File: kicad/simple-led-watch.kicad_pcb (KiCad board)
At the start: 4 copper layers, 32.8 x 32.6 mm, 169 parts, among them P1 BATTERY, P2 SWD, P3 USB_OTG, Q1 MMBT3904, Q2 MMBT3904, SW1 SPST-4PIN, SW2 SPST-4PIN, SW3 SPST-4PIN, SW4 SPST-4PIN, U1 MCP73832, U2 TPS62736, U3 STM32L052CxTx, U4 MMA8652FC, U5 USBLC6-2, U6 74HC154, Y1 32.767KHz

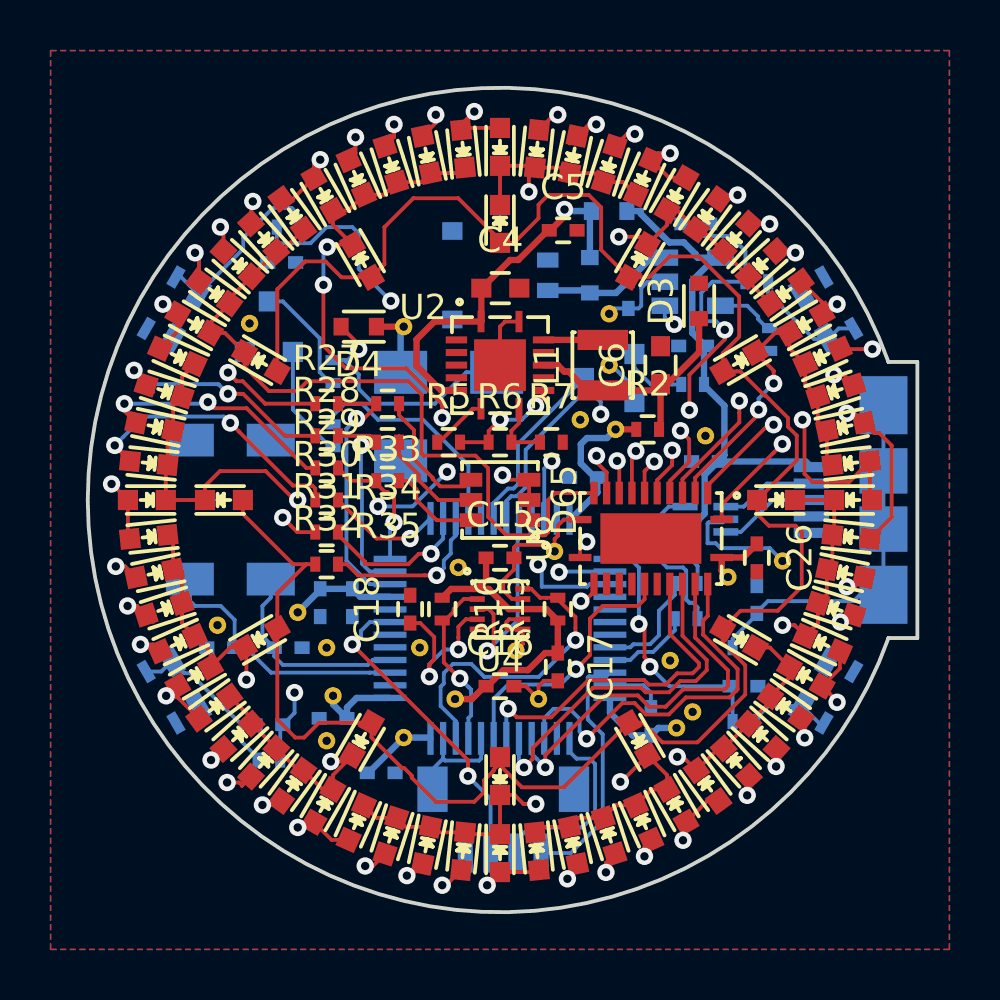
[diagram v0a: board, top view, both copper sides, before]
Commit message: Placed parts for round two
I'm pretty sure I can do it better
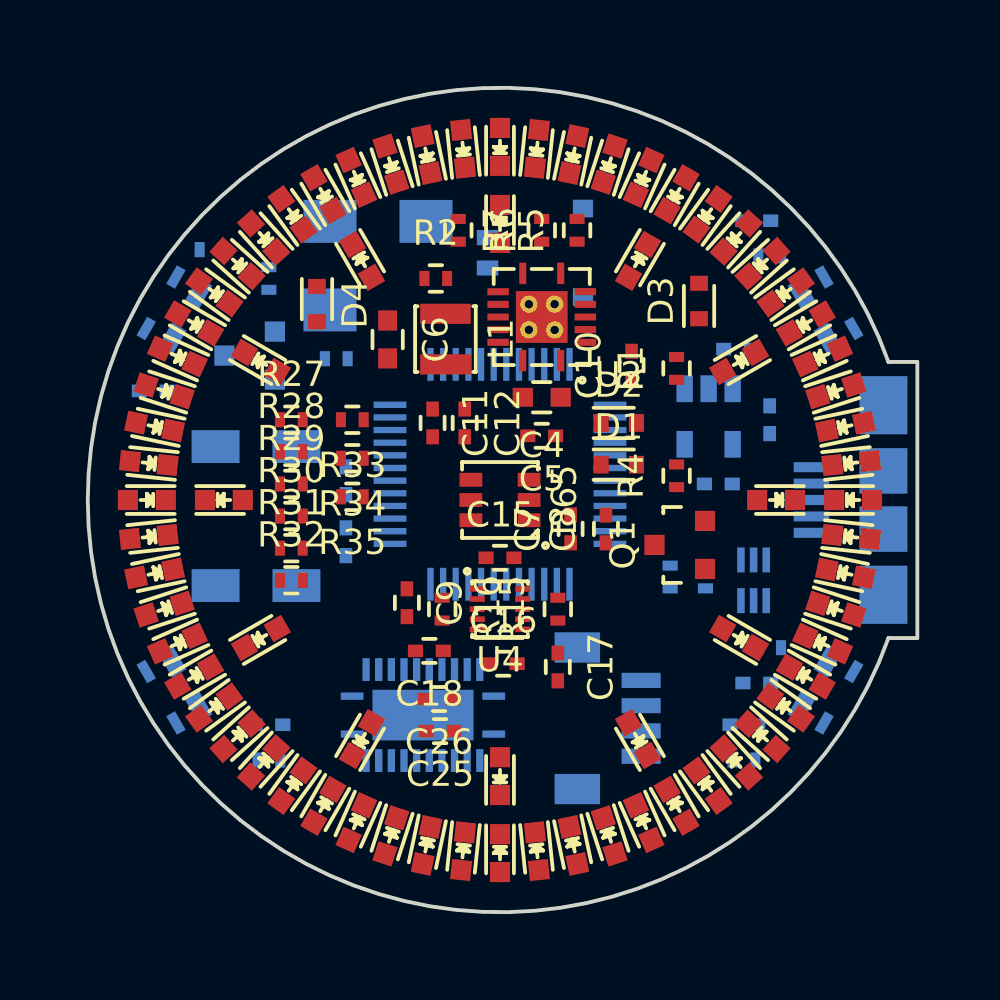
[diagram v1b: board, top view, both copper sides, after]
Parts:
- removed the REF** at (173.2, 86.4)
- removed the REF** at (165.7, 94.9)
- removed the REF** at (169.4, 81.5)
- removed the REF** at (169.4, 83.6)
- removed the REF** at (168.3, 85.7)
- removed the REF** at (176.3, 91.3)
- removed the REF** at (167.3, 90.9)
- removed the REF** at (158.2, 94.7)
- removed the REF** at (169.7, 86.1)
- removed the REF** at (172.1, 97.9)
- removed the REF** at (161.3, 98.3)
- removed the REF** at (166.6, 96.8)
- removed the REF** at (158.5, 96.6)
- removed the REF** at (163.3, 96.8)
- removed the REF** at (157.1, 93.3)
- removed the REF** at (174.1, 91.9)
- removed the REF** at (161.3, 82.0)
- removed the REF** at (161.9, 94.7)
- removed the REF** at (153.9, 93.9)
- removed the REF** at (158.2, 98.4)
- removed the REF** at (155.2, 81.9)
- removed the REF** at (172.7, 97.3)
- removed the REF** at (171.8, 95.2)
- removed the REF** at (163.4, 91.6)
- added C25: 1u, Capacitors_SMD:C_0402, F.Cu at (162.7, 98.0)
- added REF**: 1PIN_VIA, simple-led-watch:1PIN_VIA, F.Cu at (167.3, 82.2)
- added REF**: 1PIN_VIA, simple-led-watch:1PIN_VIA, F.Cu at (166.2, 82.2)
- added REF**: 1PIN_VIA, simple-led-watch:1PIN_VIA, F.Cu at (166.2, 81.2)
- added REF**: 1PIN_VIA, simple-led-watch:1PIN_VIA, F.Cu at (167.3, 81.2)
- C10, C11, C12, C7, C8, C9, D1, D2, Q1, R1, R4: moved to F.Cu
- U6: moved to B.Cu
- moved C10 18.9 mm to (170.3, 83.6), turned to 90 degrees
- moved C26 13.8 mm to (162.7, 96.8), turned to 180 degrees
- moved U6 11.4 mm to (162.1, 97.4)
- moved C6 10.8 mm to (160.7, 82.5), turned to 270 degrees
- moved R2 10.3 mm to (162.6, 80.1)
- moved D1 10.0 mm to (169.8, 87.5)
- moved R5 9.80 mm to (168.1, 78.2), turned to 90 degrees
- moved C12 9.12 mm to (163.7, 85.9)
- moved R6 8.54 mm to (163.4, 78.2), turned to 270 degrees
- moved R7 8.39 mm to (166.8, 78.2), turned to 90 degrees
- moved C5 8.17 mm to (166.8, 86.4), turned to 180 degrees
- moved C8 7.82 mm to (169.3, 90.0)
- moved C11 7.79 mm to (162.4, 85.9)
- moved C22 7.18 mm to (151.4, 84.6)
- moved Q1 7.17 mm to (172.2, 90.7), turned to 90 degrees
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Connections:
- P2 pad NC: GND -> (no net)
- Y1 pad 1: /Control/STM32_OSC32- -> /Control/STM32_OSC32+
- Y1 pad 2: /Control/STM32_OSC32+ -> /Control/STM32_OSC32-
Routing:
- net /LEDs/LED_A_R2: track 113.5 -> 0.00 mm, vias 13 -> 0
- net /LEDs/LED_A_R1: track 110.3 -> 0.00 mm, vias 13 -> 0
- net /LEDs/LED_A_R3: track 109.9 -> 0.00 mm, vias 12 -> 0
- net /LEDs/LED_A_R0: track 104.0 -> 0.00 mm, vias 7 -> 0
- net /LEDs/LED_A_R4: track 103.3 -> 0.00 mm, vias 7 -> 0
- net /LEDs/LED_A_R5: track 87.4 -> 0.00 mm
- net /LEDs/LED_SEG8: track 39.0 -> 0.00 mm, vias 2 -> 0
- net +3V3: track 38.7 -> 0.00 mm
- net GND: track 38.6 -> 0.00 mm
- net /LEDs/LED_SEG7: track 36.6 -> 0.00 mm, vias 2 -> 0
- net /LEDs/LED_SEG11: track 30.9 -> 0.00 mm, vias 4 -> 0
- net /LEDs/LED_SEG0: track 30.6 -> 0.00 mm, vias 2 -> 0
- net /LEDs/LED_SEG10: track 28.8 -> 0.00 mm
- net /Control/BTN3: track 28.8 -> 0.00 mm, vias 2 -> 0
- net /LEDs/LED_SEG9: track 28.2 -> 0.00 mm, vias 4 -> 0
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- removed copper zone on In1.Cu, net +3V3
- removed copper zone on B.Cu, net GND
- removed copper zone on F.Cu, net GND
- removed copper zone on In2.Cu, net GND
